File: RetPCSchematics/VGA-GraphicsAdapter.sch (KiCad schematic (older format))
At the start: 40 parts, among them J1 Bus_ISA_8bit, J2 74320-9004, U1 74AUC2G125, U10 ATmega644P-20PU, U11 628128, U12 628128, U13 SN74LVC245AN, U14 74LS245, U15 74LVC2G240, U16 74LVC2G240, U17 74LVC1G18, U18 74LVC1G18, U19 74LVC1G18, U2 74LVC2G240, U20 74LVC1G18, U21 ATF22V10D, U22 74LS245, U23 74LVC1G373, U24 74LVC1G373, U25 74LVC1G373, U26 74LVC1G373, U27 74LVC1G373, U28 74LVC1G373, U29 74LVC1G373, U3 ATF22V10D, U30 74LVC1G373, U31 74LVC1G373, U32 74LVC1G373, U33 74LVC1G373, U34 74LVC1G373, U36 TFP410, U37 ATF750C, U4 ATF22V10D, U5 74LS245, U6 ATF22V10D, U7 74LS245, U8 74LS245, U9 74LS245, X1 DGOF5S3

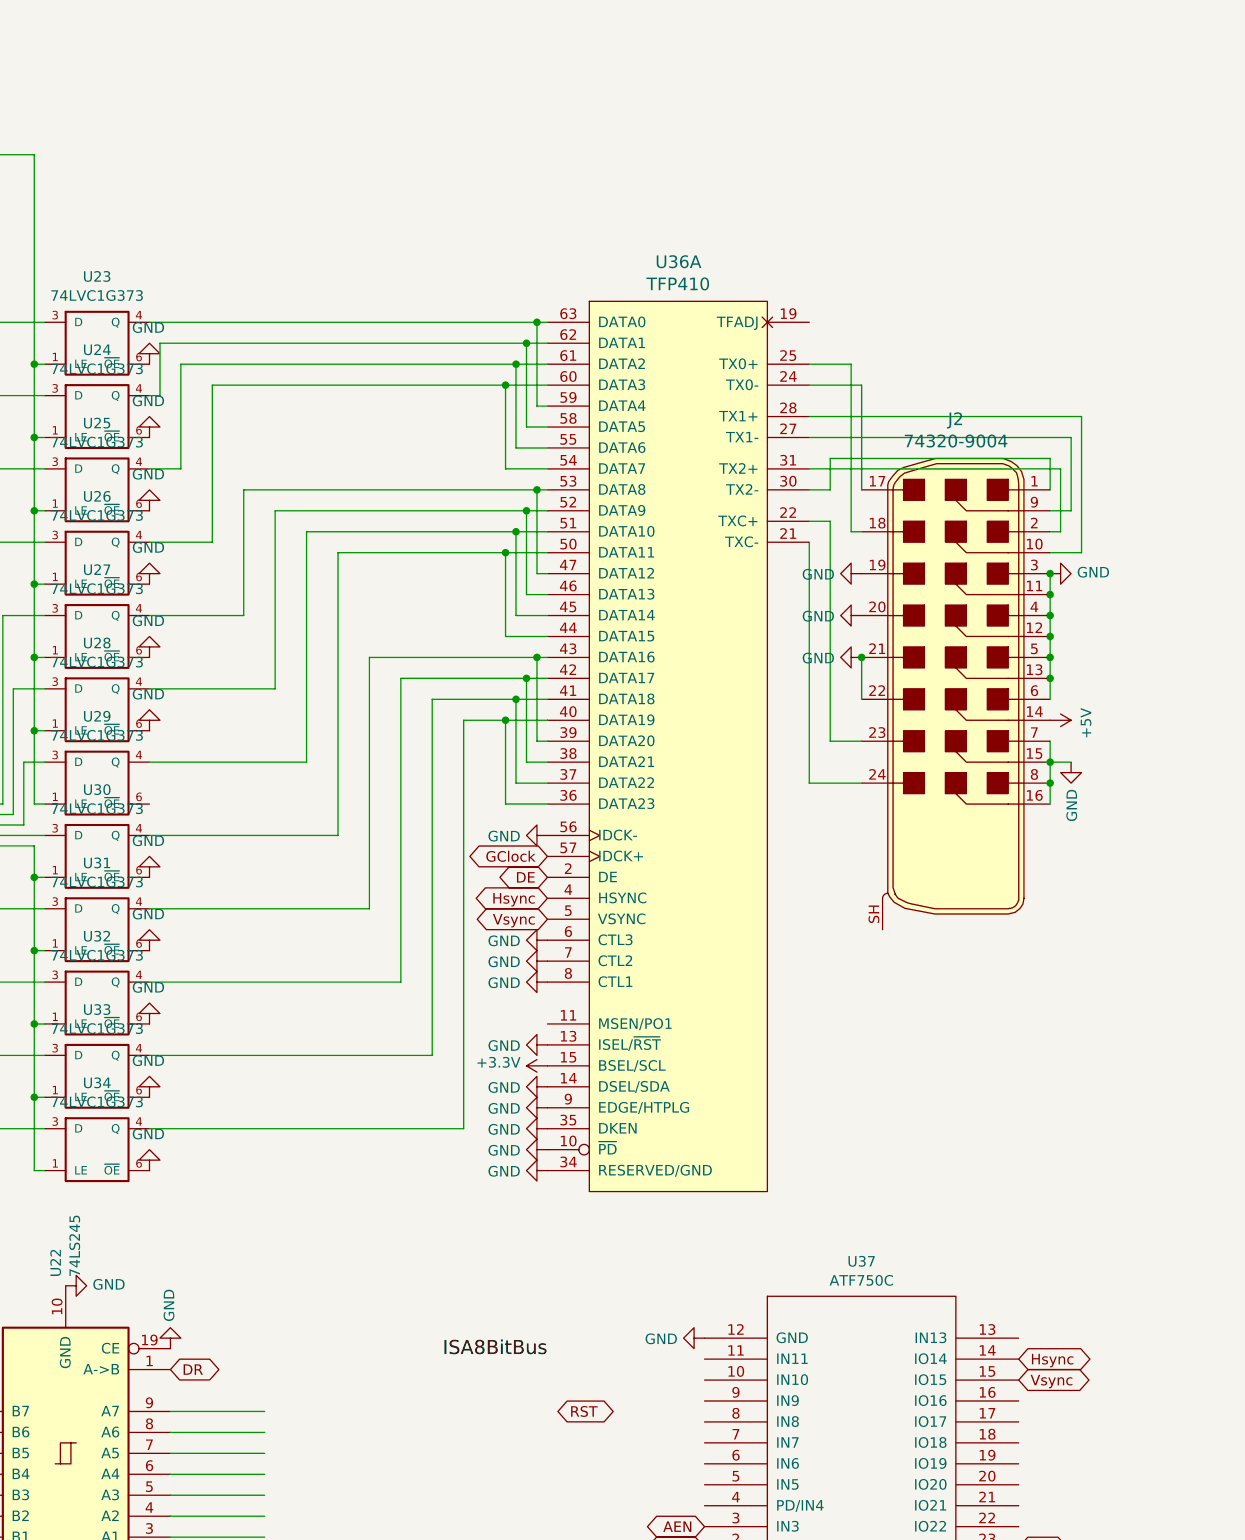
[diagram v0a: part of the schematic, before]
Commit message: sync
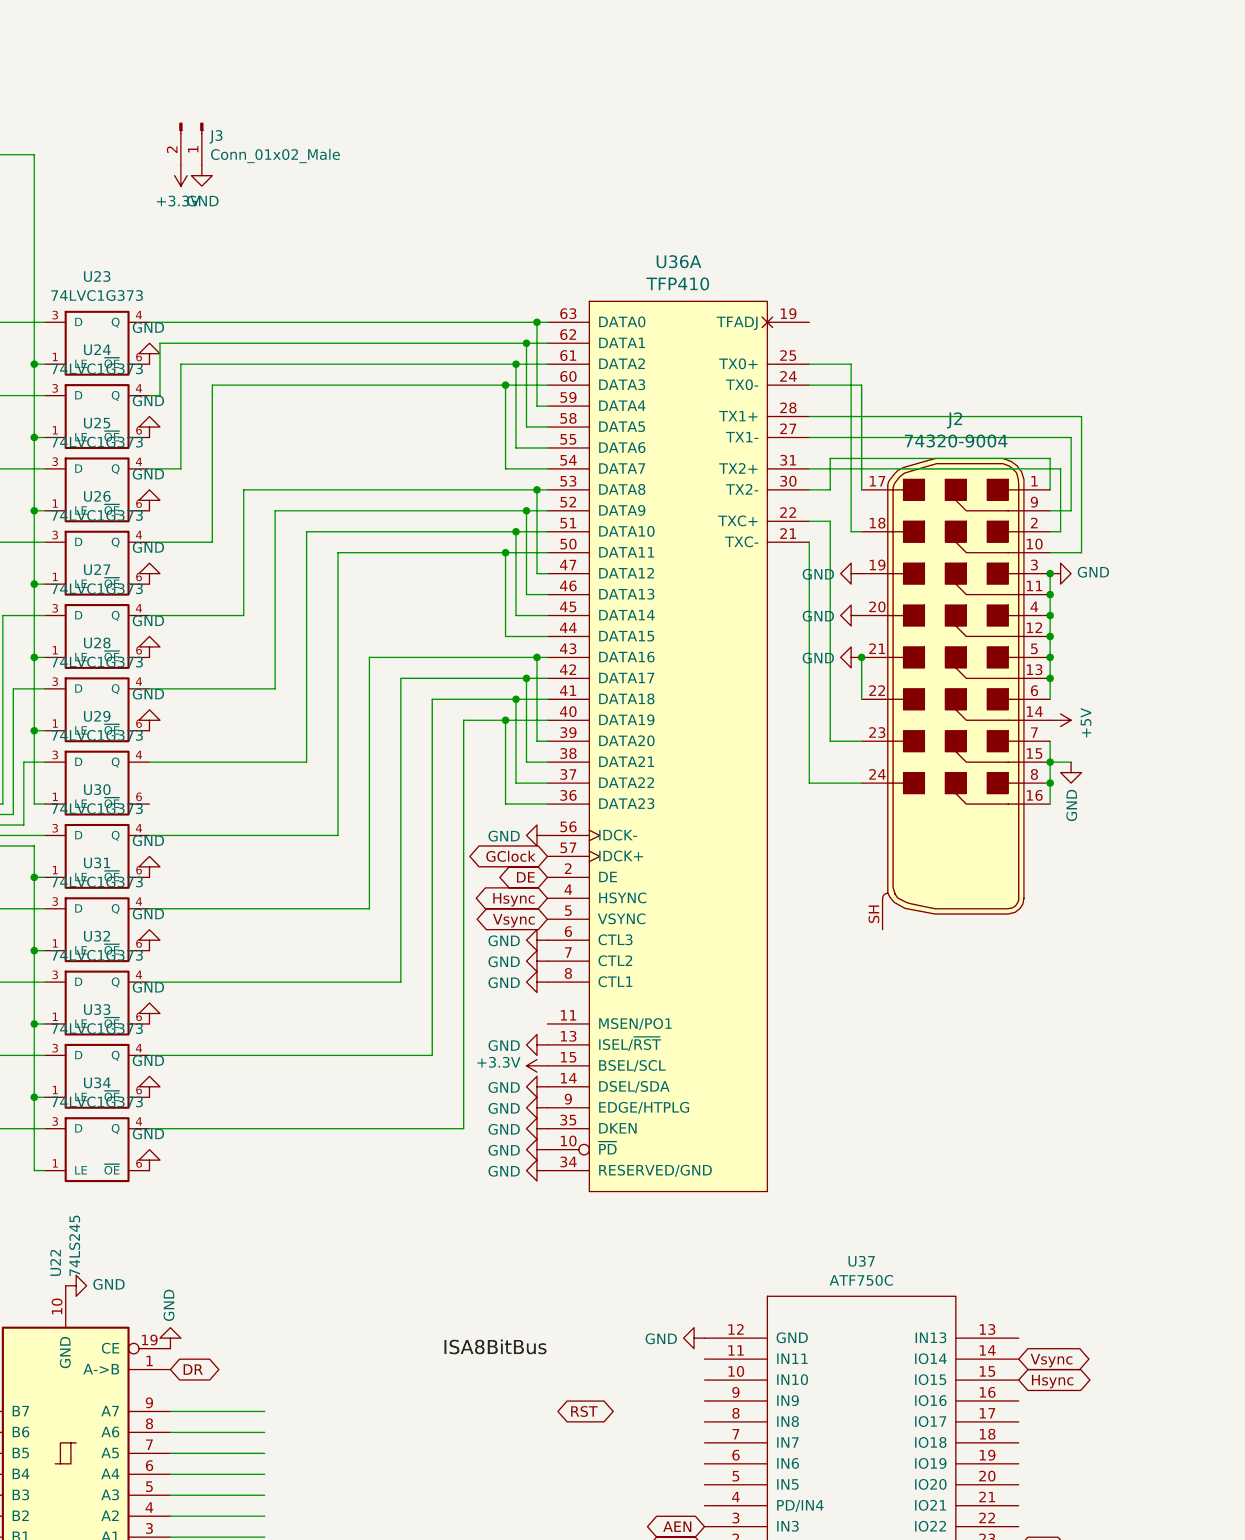
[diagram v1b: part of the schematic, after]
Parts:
- added J3: Conn_01x02_Male, Connector_PinHeader_1.00mm:PinHeader_1x02_P1.00mm_Vertical, symbol Connector:Conn_01x02_Male
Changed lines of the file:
@@
 	1    0    0    1
 $EndComp
+Text GLabel 14100 6850 2    50   BiDi ~ 0
+Hsync
 Text GLabel 14100 6750 2    50   BiDi ~ 0
-Hsync
-Text GLabel 14100 6850 2    50   BiDi ~ 0
 Vsync
 Text GLabel 11850 4550 0    50   BiDi ~ 0
@@
 D1
 Wire Bus Line
+	1650 8050 2150 8050
+Wire Bus Line
+	10350 9800 10350 11000
+Wire Wire Line
+	3900 4850 4150 4850
+Wire Wire Line
+	2550 6350 4750 6350
+Wire Wire Line
+	2650 6250 4700 6250
+Wire Wire Line
+	3850 4950 4150 4950
+Wire Wire Line
+	3800 5050 4150 5050
+Wire Wire Line
+	3750 5150 4150 5150
+Wire Wire Line
+	3700 5250 4200 5250
+Wire Wire Line
+	3650 5350 4250 5350
+Wire Wire Line
+	3600 5450 4300 5450
+Wire Wire Line
+	3550 5550 4350 5550
+Wire Wire Line
+	3300 5750 4450 5750
+Wire Wire Line
+	3350 5850 4500 5850
+Wire Wire Line
+	3400 5950 4550 5950
+Wire Wire Line
+	3450 6050 4600 6050
+Wire Wire Line
+	2750 6150 4650 6150
+Wire Wire Line
+	3500 5650 4400 5650
+Wire Bus Line
+	6650 5550 7350 5550
+Wire Bus Line
+	4050 6700 4700 6700
+Wire Bus Line
+	9850 8950 9850 9800
+Wire Bus Line
+	1850 6700 4050 6700
+Wire Bus Line
+	8050 8850 8050 9800
+Wire Bus Line
+	10350 8500 10350 9800
+Wire Bus Line
+	2150 9700 5950 9700
+Wire Bus Line
 	4050 4850 4050 6700
 Wire Bus Line
-	1650 8050 2150 8050
-Wire Wire Line
-	2550 6350 4750 6350
-Wire Wire Line
-	2650 6250 4700 6250
-Wire Wire Line
-	3850 4950 4150 4950
-Wire Wire Line
-	3800 5050 4150 5050
-Wire Wire Line
-	3750 5150 4150 5150
-Wire Wire Line
-	3700 5250 4200 5250
-Wire Wire Line
-	3650 5350 4250 5350
-Wire Wire Line
-	3600 5450 4300 5450
-Wire Wire Line
-	3550 5550 4350 5550
-Wire Wire Line
-	3300 5750 4450 5750
-Wire Wire Line
-	3350 5850 4500 5850
-Wire Wire Line
-	3400 5950 4550 5950
-Wire Wire Line
-	3450 6050 4600 6050
-Wire Wire Line
-	2750 6150 4650 6150
-Wire Wire Line
-	3500 5650 4400 5650
-Wire Bus Line
-	10350 9800 10350 11000
-Wire Wire Line
-	3900 4850 4150 4850
-Wire Bus Line
-	6650 5550 7350 5550
-Wire Bus Line
-	4050 6700 4700 6700
-Wire Bus Line
-	9850 8950 9850 9800
-Wire Bus Line
-	1850 6700 4050 6700
-Wire Bus Line
-	8050 8850 8050 9800
-Wire Bus Line
-	10350 8500 10350 9800
-Wire Bus Line
-	2150 9700 5950 9700
-Wire Bus Line
 	3400 11000 10350 11000
 Wire Bus Line
@@
 Wire Bus Line
 	2150 8000 5850 8000
+$Comp
+L Connector:Conn_01x02_Male J3
+U 1 1 5C554E39
+P 10200 850
+F 0 "J3" V 10260 890 50  0000 L CNN
+F 1 "Conn_01x02_Male" V 10351 890 50  0000 L CNN
+F 2 "Connector_PinHeader_1.00mm:PinHeader_1x02_P1.00mm_Vertical" H 10200 850 50  0001 C CNN
+F 3 "~" H 10200 850 50  0001 C CNN
+	1    10200 850
+	0    1    1    0
+$EndComp
+$Comp
+L power:+3.3V #PWR0102
+U 1 1 5C554FE5
+P 10100 1050
+F 0 "#PWR0102" H 10100 900 50  0001 C CNN
+F 1 "+3.3V" H 10115 1223 50  0000 C CNN
+F 2 "" H 10100 1050 50  0001 C CNN
+F 3 "" H 10100 1050 50  0001 C CNN
+	1    10100 1050
+	-1   0    0    1
+$EndComp
+$Comp
+L power:GND #PWR0103
+U 1 1 5C5550EF
+P 10200 1050
+F 0 "#PWR0103" H 10200 800 50  0001 C CNN
+F 1 "GND" H 10205 877 50  0000 C CNN
+F 2 "" H 10200 1050 50  0001 C CNN
+F 3 "" H 10200 1050 50  0001 C CNN
+	1    10200 1050
+	1    0    0    -1
+$EndComp
 $EndSCHEMATC
